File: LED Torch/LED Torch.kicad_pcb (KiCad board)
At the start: 2 copper layers, 4 parts, among them SW1 SW_Push

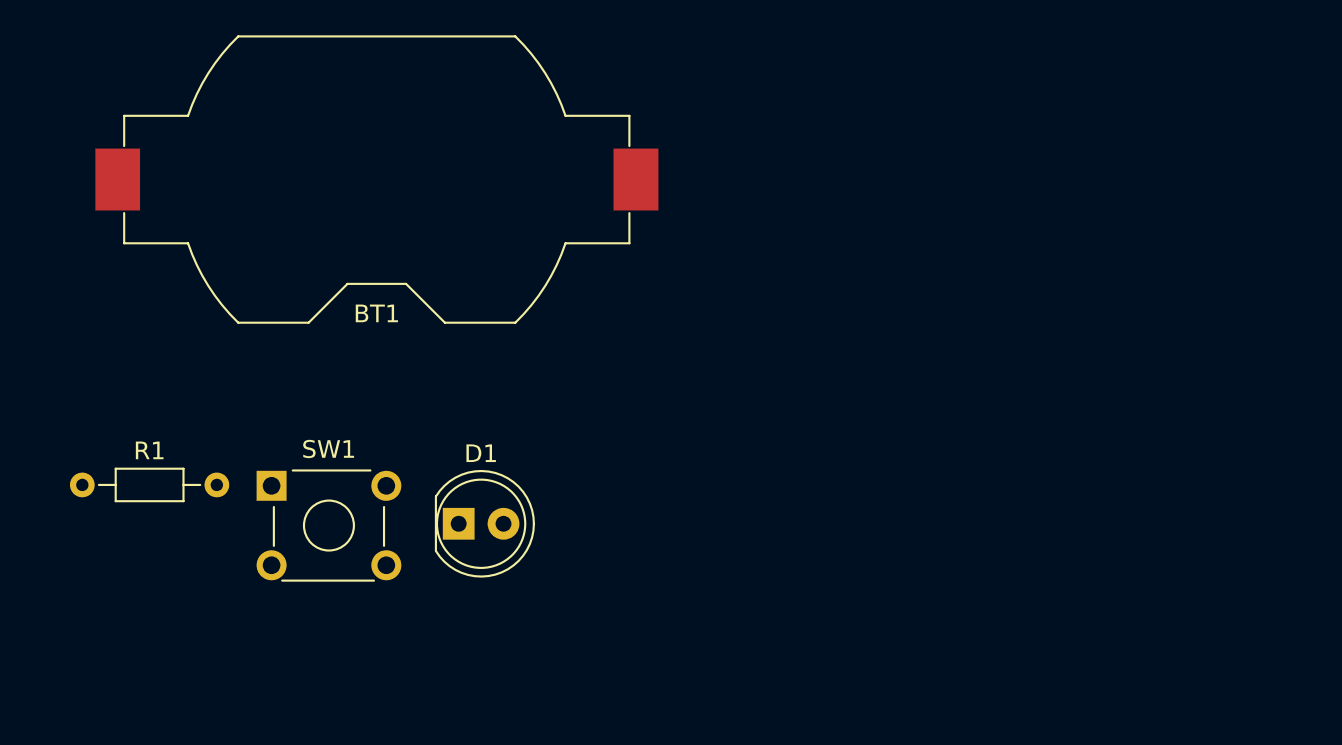
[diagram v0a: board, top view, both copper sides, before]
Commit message: basic layout
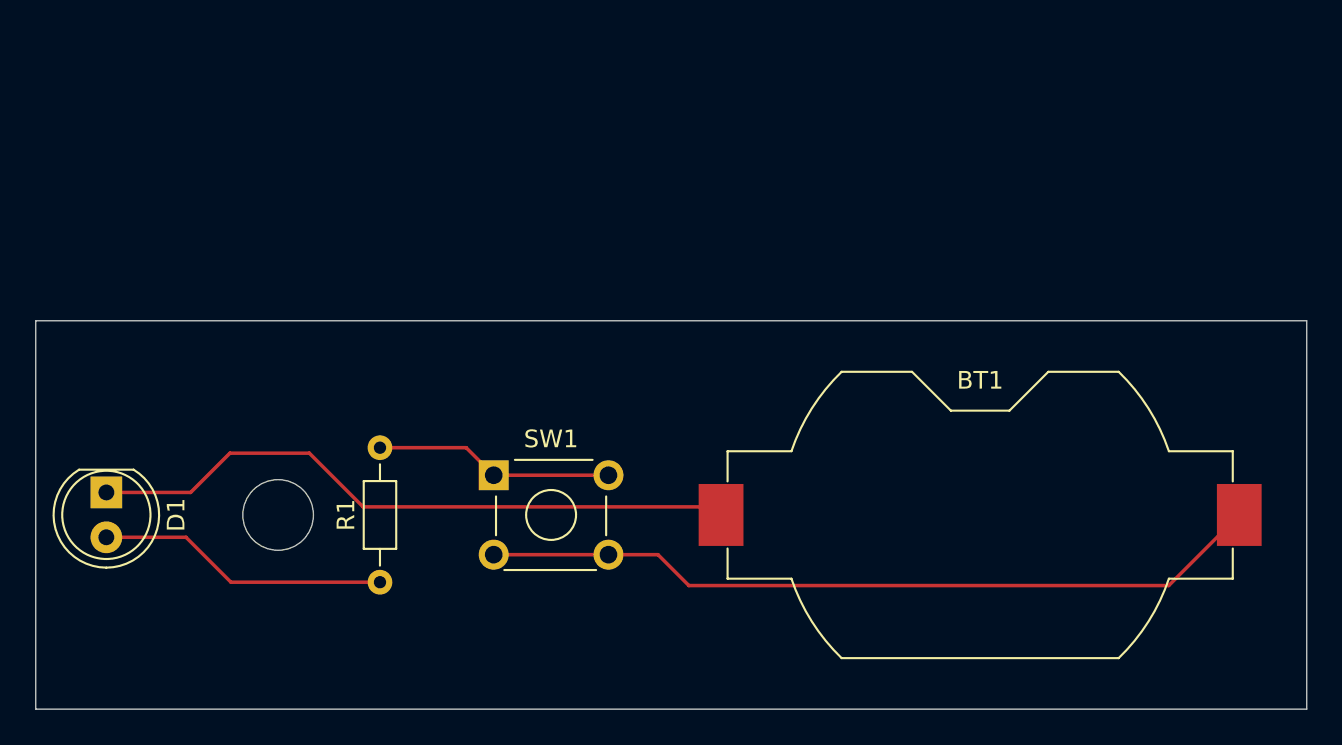
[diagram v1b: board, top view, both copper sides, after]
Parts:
- moved BT1 39.1 mm to (177.5, 100.0), turned to 180 degrees
- moved D1 20.0 mm to (128.0, 98.7), turned to -90 degrees
- moved R1 17.7 mm to (143.5, 103.8), turned to 90 degrees
- moved SW1 12.6 mm to (149.9, 97.8)
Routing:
- net /VCC: track 0.00 -> 44.6 mm
- net /GND: track 0.00 -> 37.2 mm
- net Net-(D1-A): track 0.00 -> 16.6 mm
- net Net-(R1-Pad2): track 0.00 -> 13.6 mm
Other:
- board outline added: 72 x 22 mm
